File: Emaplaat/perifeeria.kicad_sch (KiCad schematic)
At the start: 28 parts, among them J3 Conn_01x05_Socket, Q1 2N7002K

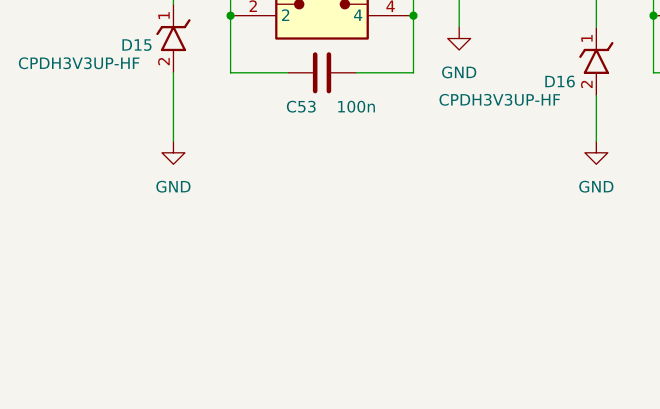
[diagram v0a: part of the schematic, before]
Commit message: natuke parandusi
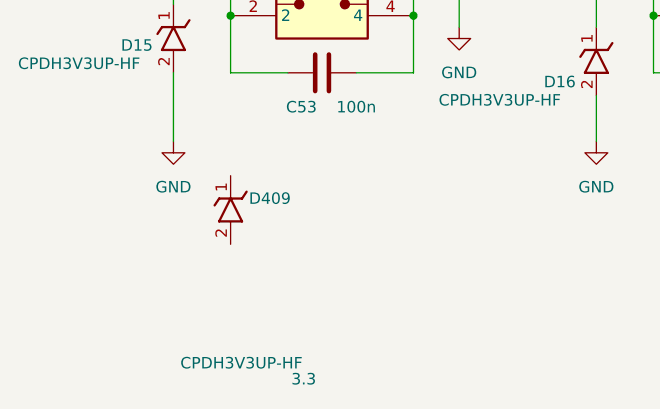
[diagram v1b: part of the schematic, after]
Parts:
- added D409: CPDH3V3UP-HF, Diode_SMD:D_SOD-523, symbol CPDH3V3UP-HF:CPDH3V3UP-HF
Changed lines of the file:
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@@
+	)
+	(symbol
+		(lib_name "CPDH3V3UP-HF_2")
+		(lib_id "CPDH3V3UP-HF:CPDH3V3UP-HF")
+		(at 57.15 165.1 270)
+		(unit 1)
+		(exclude_from_sim no)
+		(in_bom yes)
+		(on_board yes)
+		(dnp no)
+		(property "Reference" "D409"
+			(at 59.182 172.72 90)
+			(effects
+				(font
+					(size 1.27 1.27)
+				)
+				(justify left)
+			)
+		)
+		(property "Value" "CPDH3V3UP-HF"
+			(at 51.562 191.008 90)
+			(effects
+				(font
+					(size 1.27 1.27)
+				)
+				(justify left)
+			)
+		)
+		(property "Footprint" "Diode_SMD:D_SOD-523"
+			(at -36.5 175.26 0)
+			(effects
+				(font
+					(size 1.27 1.27)
+				)
+				(justify left bottom)
+				(hide yes)
+			)
+		)
+		(property "Datasheet" "https://datasheet.datasheetarchive.com/originals/distributors/Datasheets-DGA26/1842371.pdf"
+			(at -136.5 175.26 0)
+			(effects
+				(font
+					(size 1.27 1.27)
+				)
+				(justify left bottom)
+				(hide yes)
+			)
+		)
+		(property "Description" "ESD Suppressors / TVS Diodes 5.5V, 15Kv"
+			(at 70.866 164.846 0)
+			(effects
+				(font
+					(size 1.27 1.27)
+				)
+				(hide yes)
+			)
+		)
+		(property "Height" "0.77"
+			(at -336.5 175.26 0)
+			(effects
+				(font
+					(size 1.27 1.27)
+				)
+				(justify left bottom)
+				(hide yes)
+			)
+		)
+		(property "Mouser Part Number" "750-CPDH3V3UP-HF"
+			(at -436.5 175.26 0)
+			(effects
+				(font
+					(size 1.27 1.27)
+				)
+				(justify left bottom)
+				(hide yes)
+			)
+		)
+		(property "Mouser Price/Stock" "https://www.mouser.co.uk/ProductDetail/Comchip-Technology/CPDH3V3UP-HF?qs=XEIV%2Fho1H6em2DT135enQw%3D%3D"
+			(at -536.5 175.26 0)
+			(effects
+				(font
+					(size 1.27 1.27)
+				)
+				(justify left bottom)
+				(hide yes)
+			)
+		)
+		(property "Manufacturer_Name" "Comchip Technology"
+			(at -636.5 175.26 0)
+			(effects
+				(font
+					(size 1.27 1.27)
+				)
+				(justify left bottom)
+				(hide yes)
+			)
+		)
+		(property "Manufacturer_Part_Number" "CPDH3V3UP-HF"
+			(at -736.5 175.26 0)
+			(effects
+				(font
+					(size 1.27 1.27)
+				)
+				(justify left bottom)
+				(hide yes)
+			)
+		)
+		(property "Voltage" "3.3"
+			(at 65.278 192.786 90)
+			(effects
+				(font
+					(size 1.27 1.27)
+				)
+			)
+		)
+		(pin "2"
+		)
+		(pin "1"
+		)
+		(instances
+			(project "Emaplaat"
+				(path "/489224c0-ace1-4530-aa61-a5d03adf1434/ac5852bd-1625-445e-9b6b-b65a0daab019"
+					(reference "D409")
+					(unit 1)
+				)
+			)
+		)
 	)
 	(symbol
